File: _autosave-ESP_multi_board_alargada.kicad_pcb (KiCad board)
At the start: 2 copper layers, 24 parts, among them P101 CONN_01X02, P102 CONN_01X06, P103 CONN_01X02, P104 CONN_01X06, P105 CONN_01X12, P106 CONN_01X03, P107 CONN_I2C_MPU6050, P108 CONN_PINES_DIG, SW101 SW_PUSH_SMALL, SW102 SWITCH_INV, U1 LD1117S33TR, U101 L293DD, U102 ESP-12, U103 MAX11605EEE+, U104 MCP23008

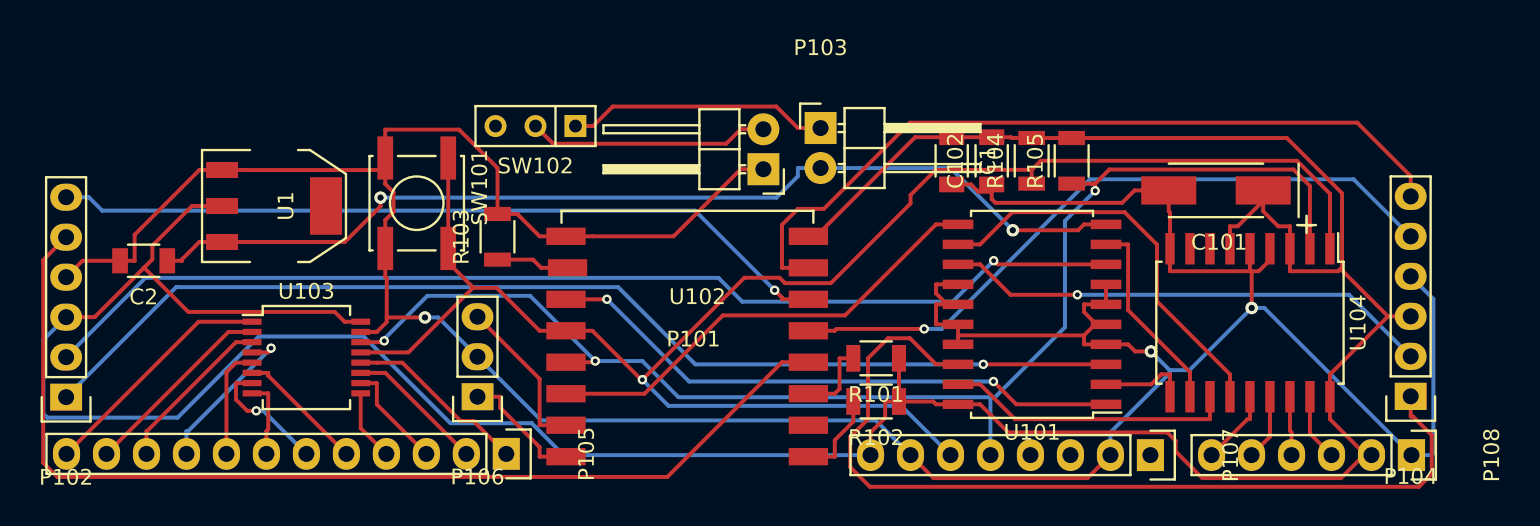
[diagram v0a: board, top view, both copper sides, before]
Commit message: routing
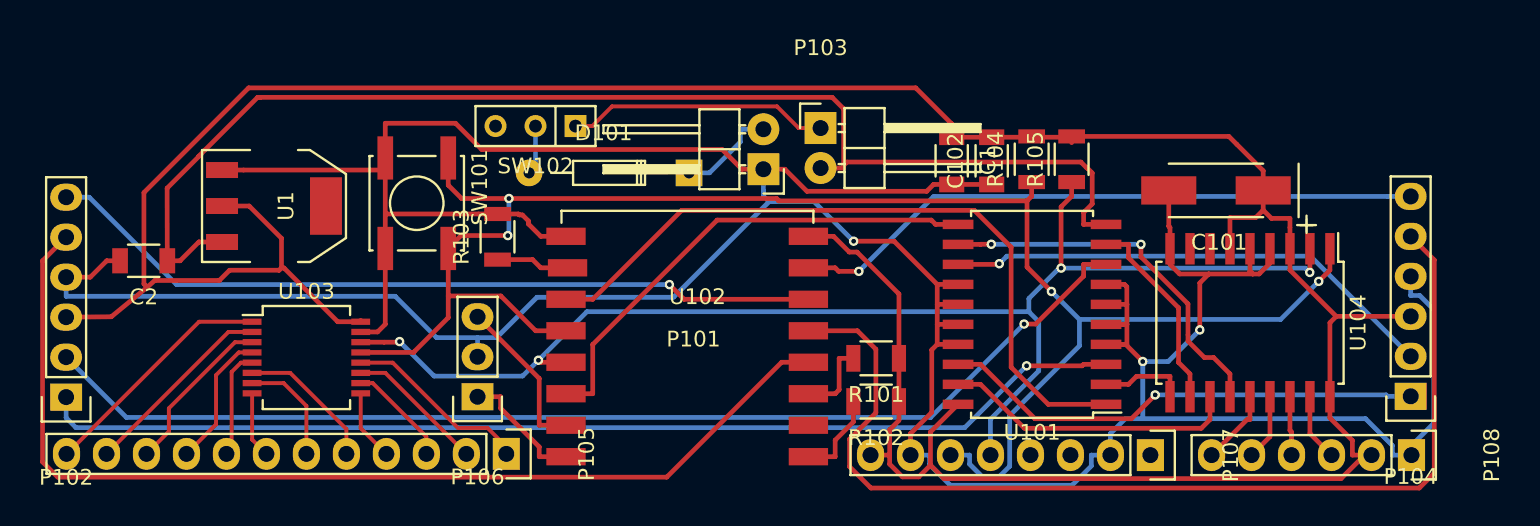
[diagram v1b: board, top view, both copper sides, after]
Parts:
- added D101: D, Diodes_ThroughHole:Diode_DO-35_SOD27_Horizontal_RM10, F.Cu at (167.1, 75.9)
- moved R104 0.10 mm to (188.9, 75.1)
- moved R105 0.10 mm to (191.4, 75.1)
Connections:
- P101 pad 2: Net-(P101-Pad2) -> Net-(D101-Pad1)
- SW102 pad 2: Net-(P101-Pad2) -> Net-(D101-Pad2)
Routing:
- net GND: track 221.7 -> 256.0 mm
- net M2+: track 57.7 -> 30.8 mm, vias 0 -> 1
- net ENC2_A: track 44.5 -> 67.4 mm, vias 1 -> 0
- net VCC: track 64.5 -> 80.6 mm, vias 2 -> 0
- net Net-(P101-Pad2): track 15.3 -> 0.00 mm
- net EN1: track 36.4 -> 45.5 mm, vias 2 -> 0
- net VDD: track 207.9 -> 199.3 mm
- net ENC2_B: track 49.0 -> 41.0 mm, vias 0 -> 1
- net Net-(D101-Pad1): track 0.00 -> 6.35 mm
- net Net-(D101-Pad2): track 0.00 -> 3.14 mm
- net SCL: track 107.8 -> 110.5 mm, vias 1 -> 4
- net M1-: track 70.0 -> 72.1 mm
- net EN2: track 28.7 -> 30.7 mm
- net M2_B: track 25.9 -> 24.0 mm, vias 0 -> 2
- net Net-(P105-Pad9): track 10.4 -> 8.67 mm, vias 1 -> 0
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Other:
- net class Default: trace_width 0.25 -> 0.3
- net class power: trace_width 0.25 -> 0.3
- net class small added: clearance 0.25, trace_width 0.25, via_dia 0.6, via_drill 0.4
- net class special added: clearance 0.2, trace_width 0.3, via_dia 0.6, via_drill 0.4
- net class special+ added: clearance 0.15, trace_width 0.3, via_dia 0.6, via_drill 0.4
